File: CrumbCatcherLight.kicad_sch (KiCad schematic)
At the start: 16 parts, among them J1 USB_C_Receptacle, J2 Battery with NTC, J3 Battery No NTC, J4 NTC, J5 Qi Charger In, U1 ECMF02-2AMX6, U2 PCB

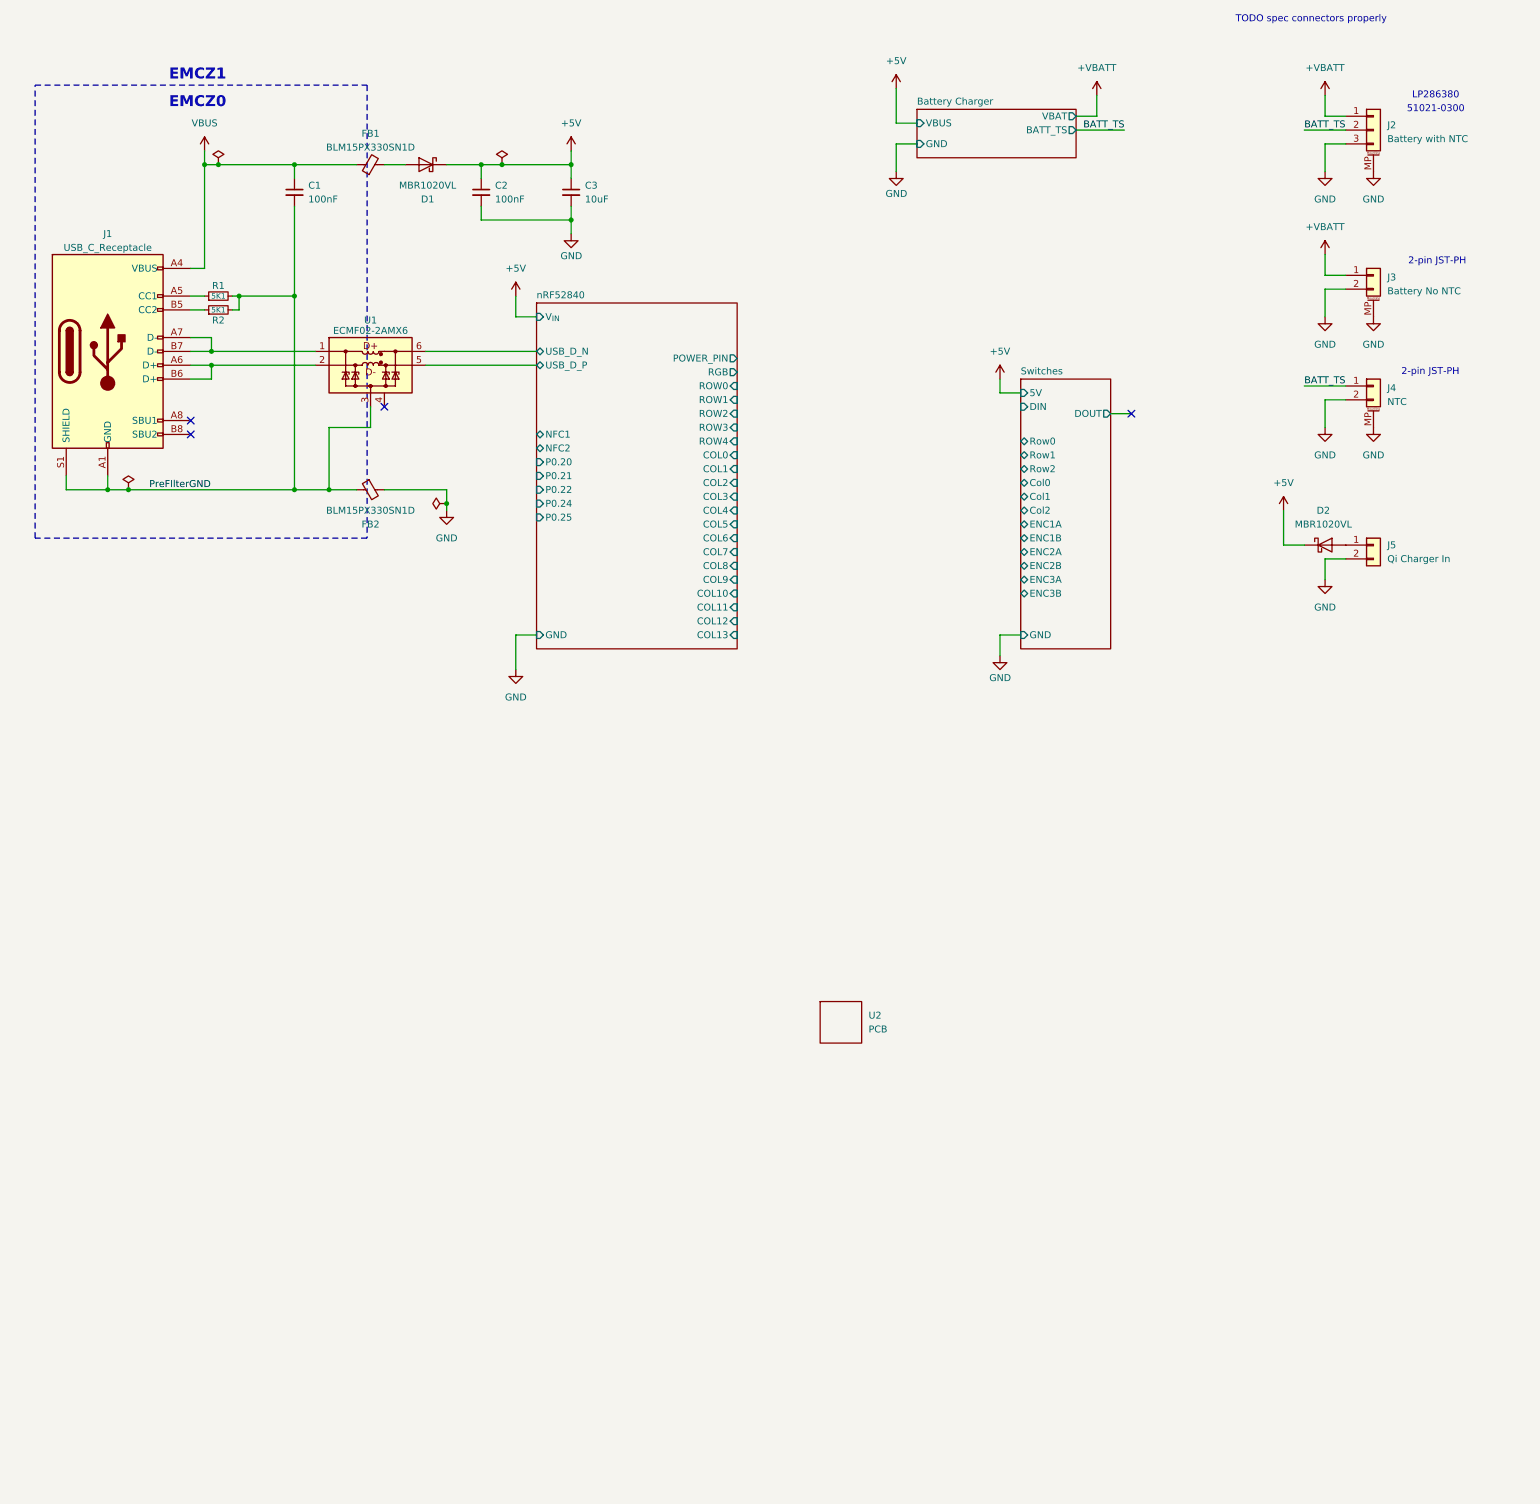
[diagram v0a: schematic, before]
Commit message: Update BOM
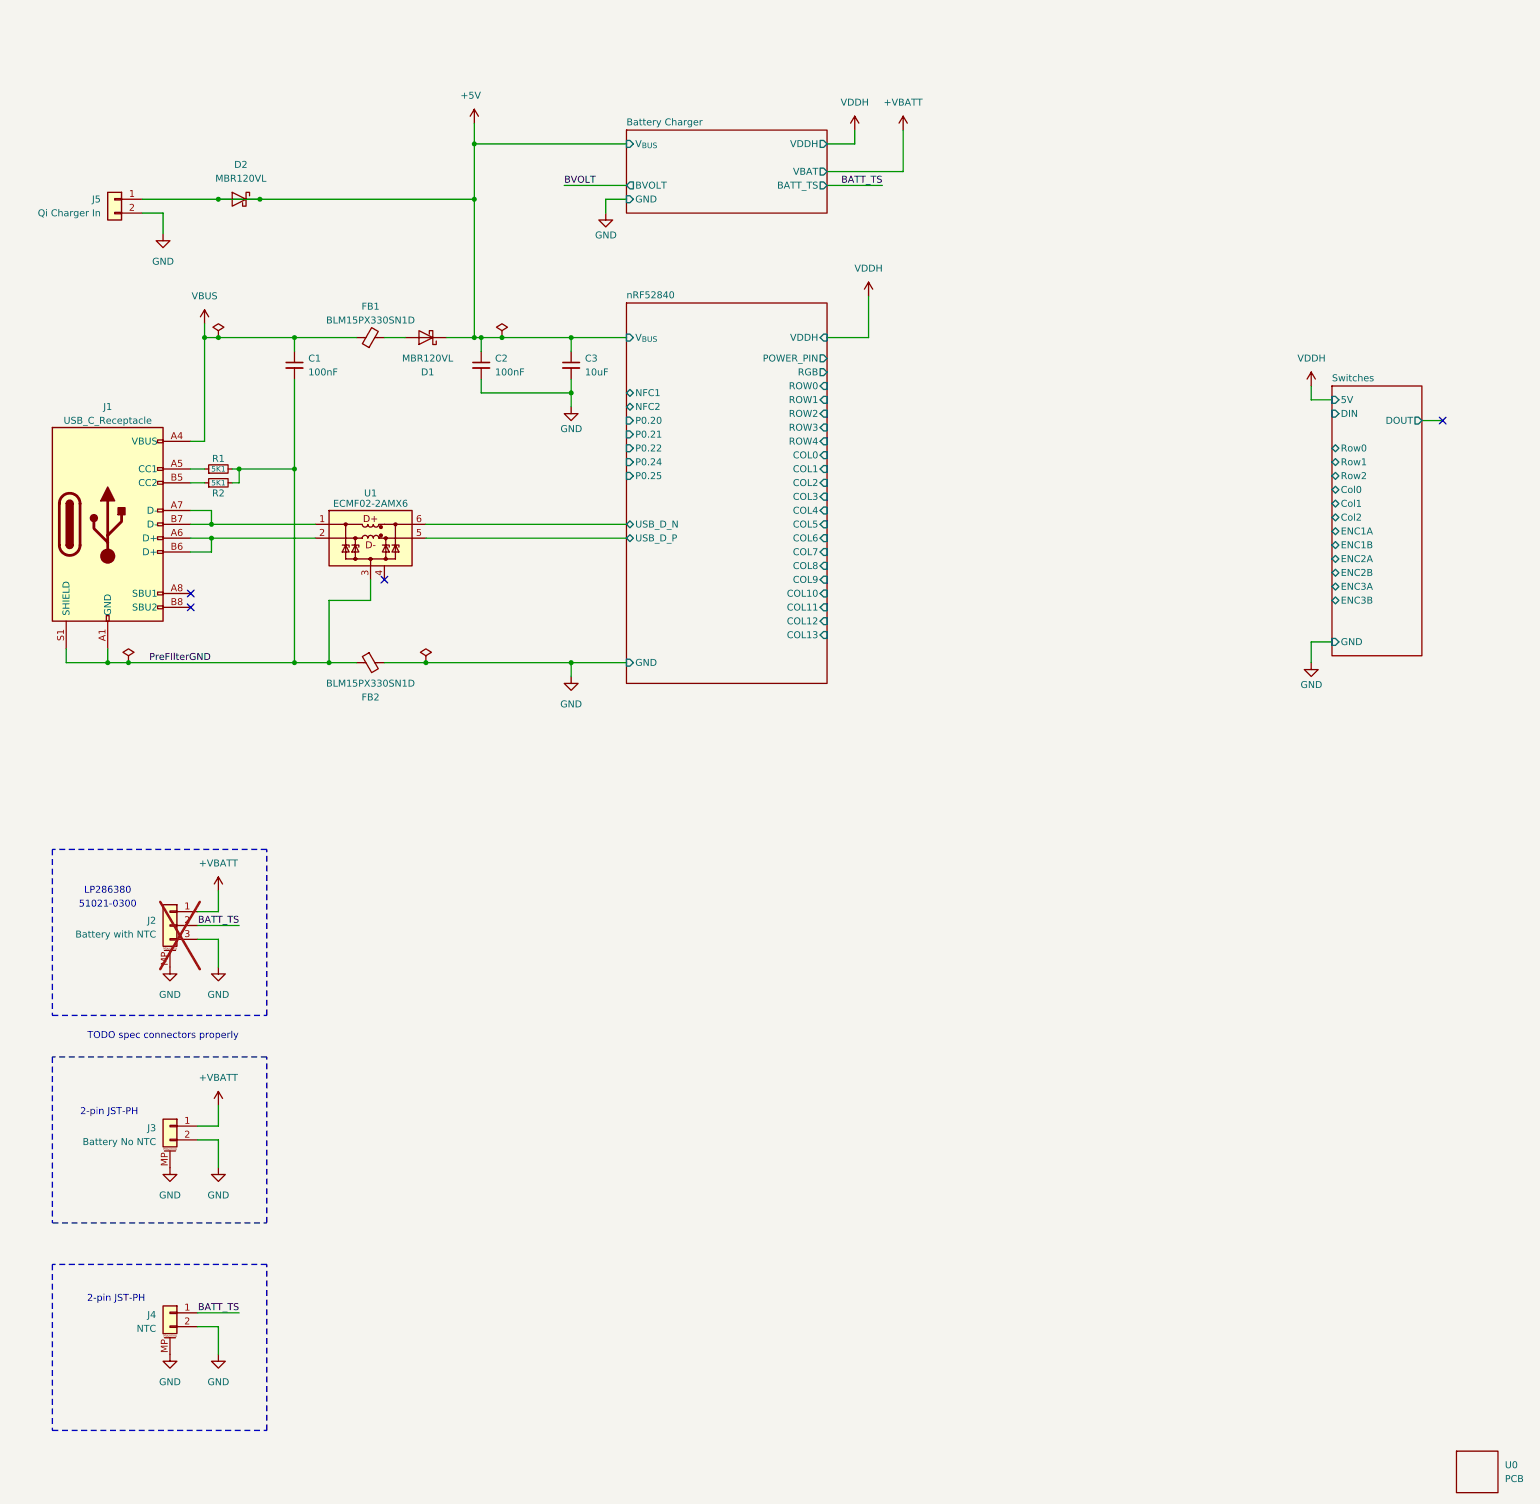
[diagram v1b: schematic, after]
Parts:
- C1, C2: footprint Capacitor_SMD:C_0402_1005Metric -> Capacitor_SMD:C_0603_1608Metric; LCSC (none) -> C432917; MPN CC0402KPX7R9BB104 -> CC0603KPX7R9BB104; Price $0.17 -> $0.10; Rating CAP 0402 50V 100 NF X7R -> CAP CER 0.1UF 50V X7R 0603; Supplier PN 13-CC0402KPX7R9BB104CT-ND -> (none); digikey (none) -> 311-3567-1-ND; mouser (none) -> 603-CC603KPX7R9BB104
- D1, D2: value MBR1020VL -> MBR120VL; MPN (none) -> MBR120VLSFT1G; Manufacturer (none) -> onsemi; Price (none) -> $0.41; Rating (none) -> DIODE SCHOTTKY 20V 1A SOD123FL; Supplier (none) -> Digikey; digikey (none) -> MBR120VLSFT1GOSCT-ND
- J2: now not fitted
- renumbered U2 to U0
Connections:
- net +5V: now also D2.2 (A), J5.1 (Pin_1)
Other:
- sheet Battery Charger ports: added BVOLT, VDDH, V_{BUS}; removed VBUS
- sheet nRF52840 ports: added VDDH, V_{BUS}; removed V_{IN}
- note removed: "EMCZ0"
- note removed: "EMCZ1"
- moved on the sheet: C3, D2, FB1, FB2, J1, J3, J4, J5, R1, R2, U0, U1
